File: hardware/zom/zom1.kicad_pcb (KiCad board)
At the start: 2 copper layers, 51.6 x 75.9 mm, 39 parts, among them J1 REG:3V3, J10 LBD, J11 uart, J12 dht22, J13 9602-a, J14 satx, J15 misc, J16 LBO, J19 9602-b, J2 prog, J3 VINS, J4 sdcard, J5 i2c-a, J6 REG:5V, J7 ANT, J8 i2c-c, J9 1wire, Q1 Q_NPN_CBE, Q2 Q_NPN_CBE, SW1 SW_Push, SW2 SW_Push, U1 ESP32-WROOM, U2 RFM95HW

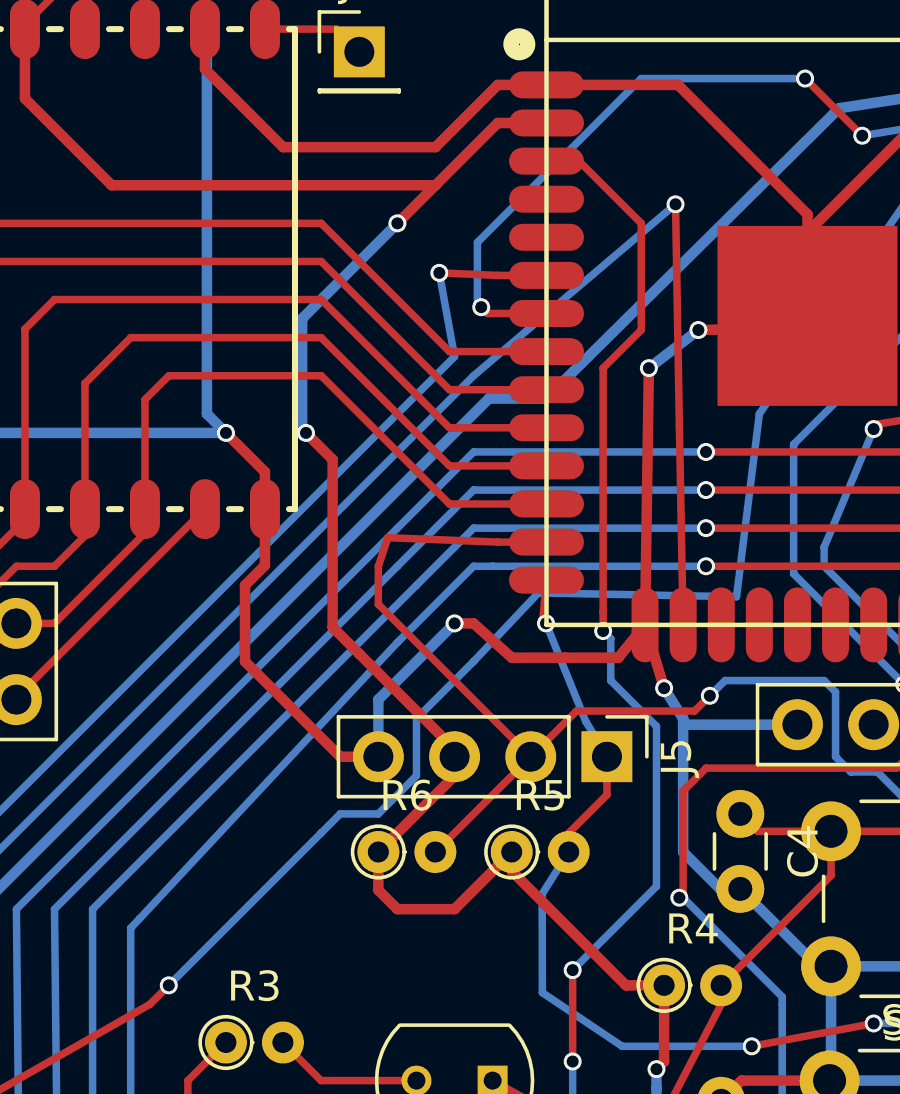
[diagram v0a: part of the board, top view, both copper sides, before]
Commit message: update
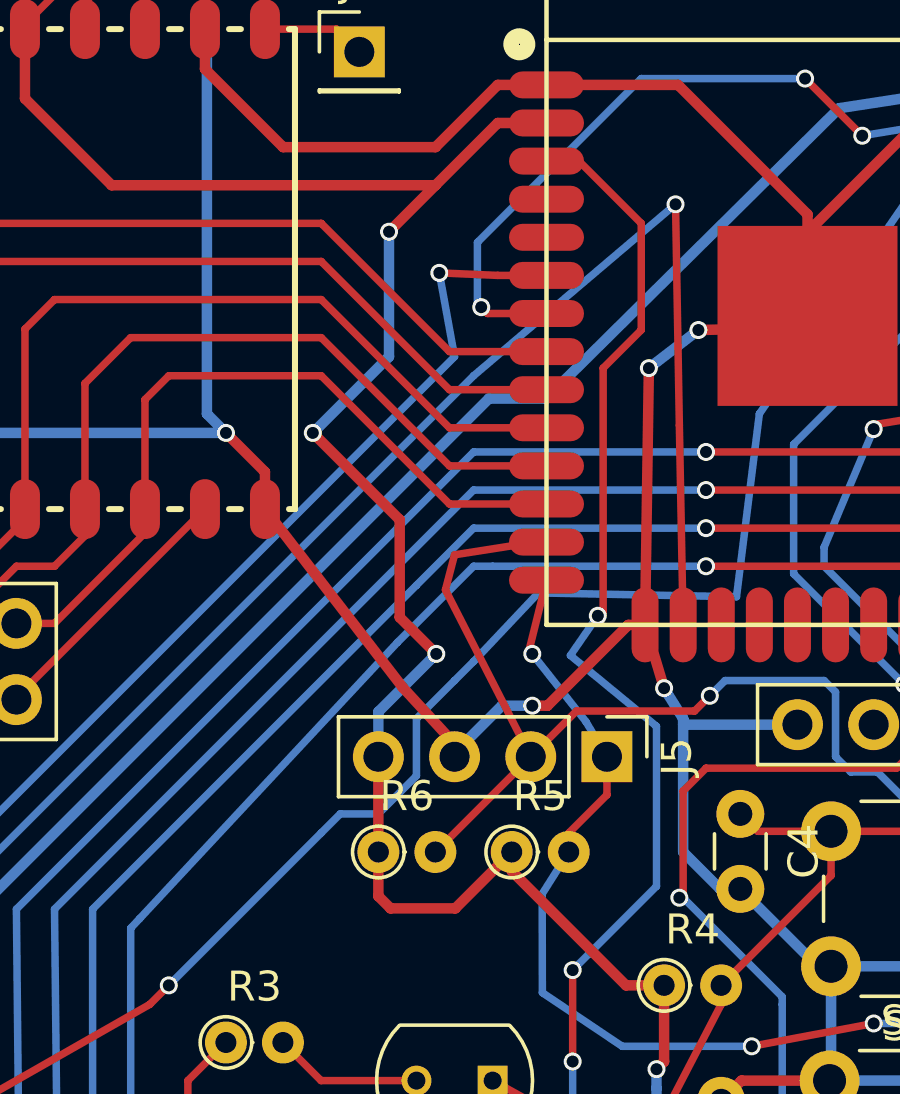
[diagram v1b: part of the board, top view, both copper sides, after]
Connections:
- J5 pad 3: +3V3 -> GND
- J5 pad 4: GND -> +3V3
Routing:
- net 14/SCL: track 56.5 -> 52.3 mm
- net GND: track 311.6 -> 307.9 mm
- net +3V3: track 200.2 -> 198.8 mm, vias 6 -> 7
- net RESET: track 63.1 -> 64.1 mm
